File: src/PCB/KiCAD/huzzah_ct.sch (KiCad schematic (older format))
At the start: 6 parts, among them CON1 BARREL_JACK, U1 MCP3008, U2 DS18B20, U3 Adafruit_HUZZAH, U4 LM317T

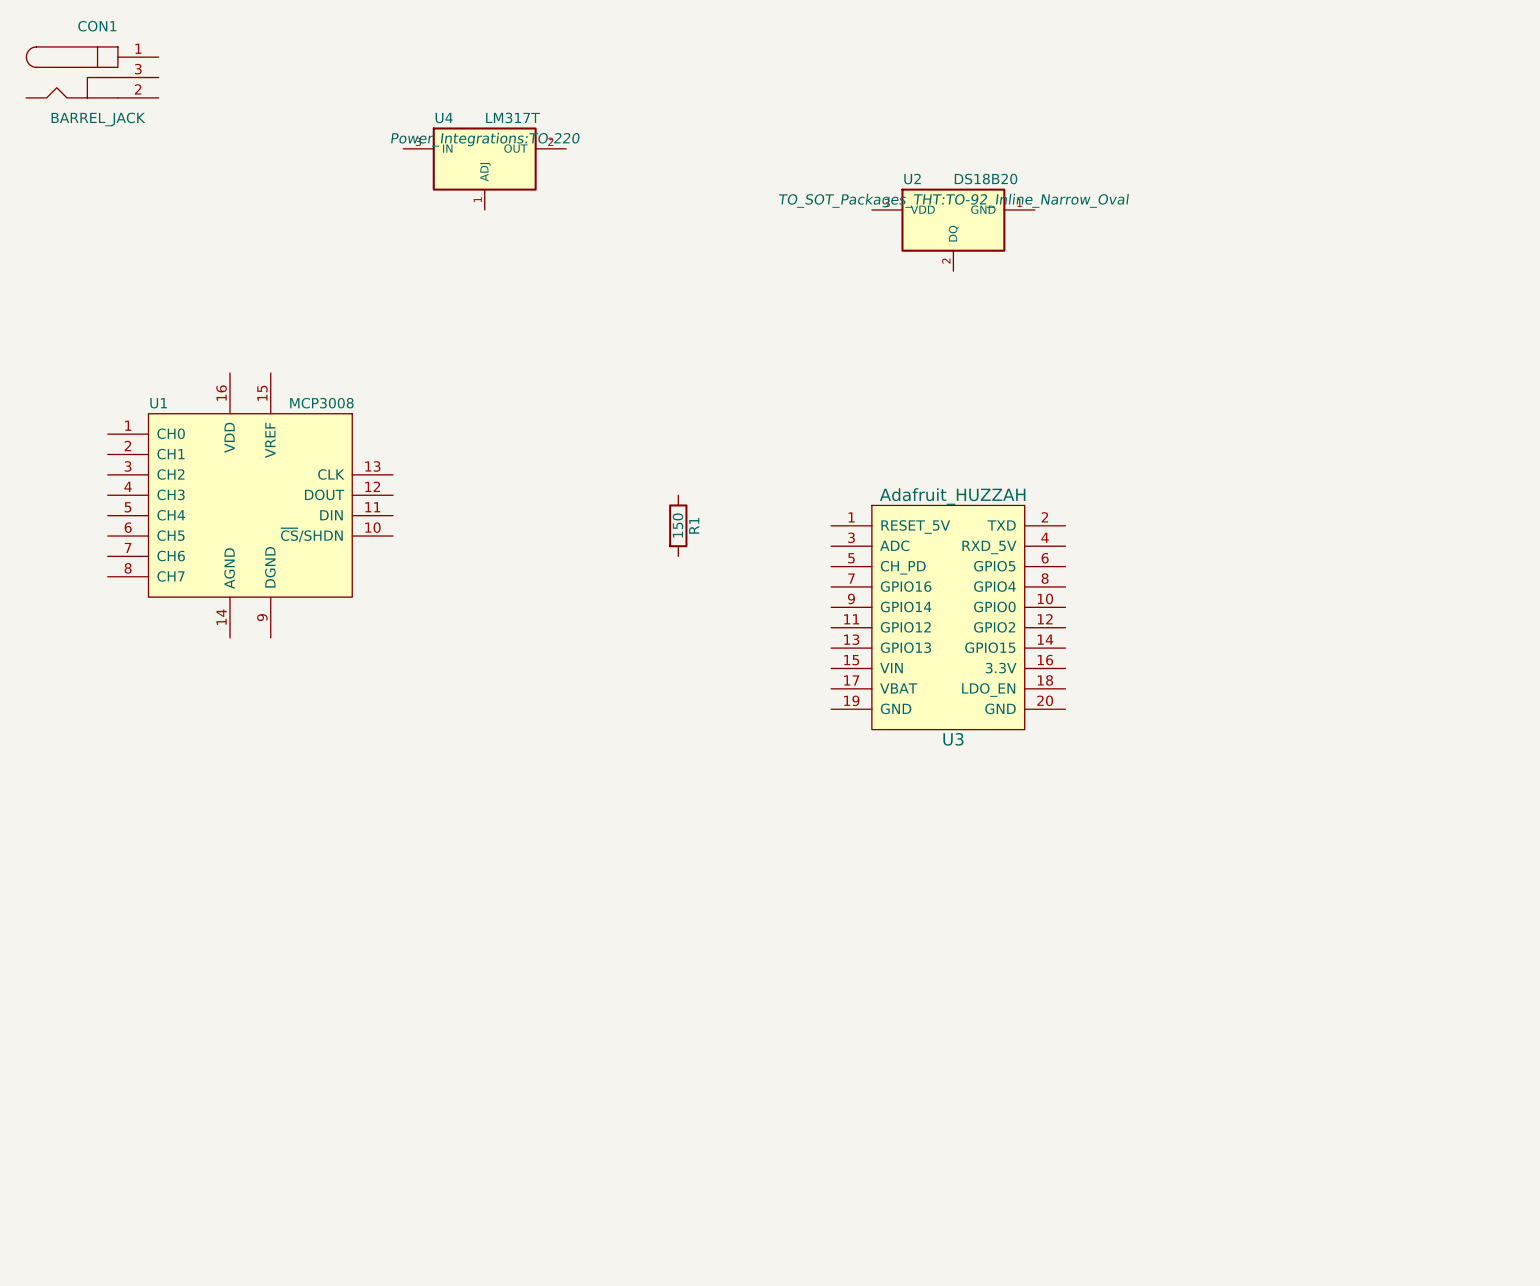
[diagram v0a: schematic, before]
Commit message: pcb routing
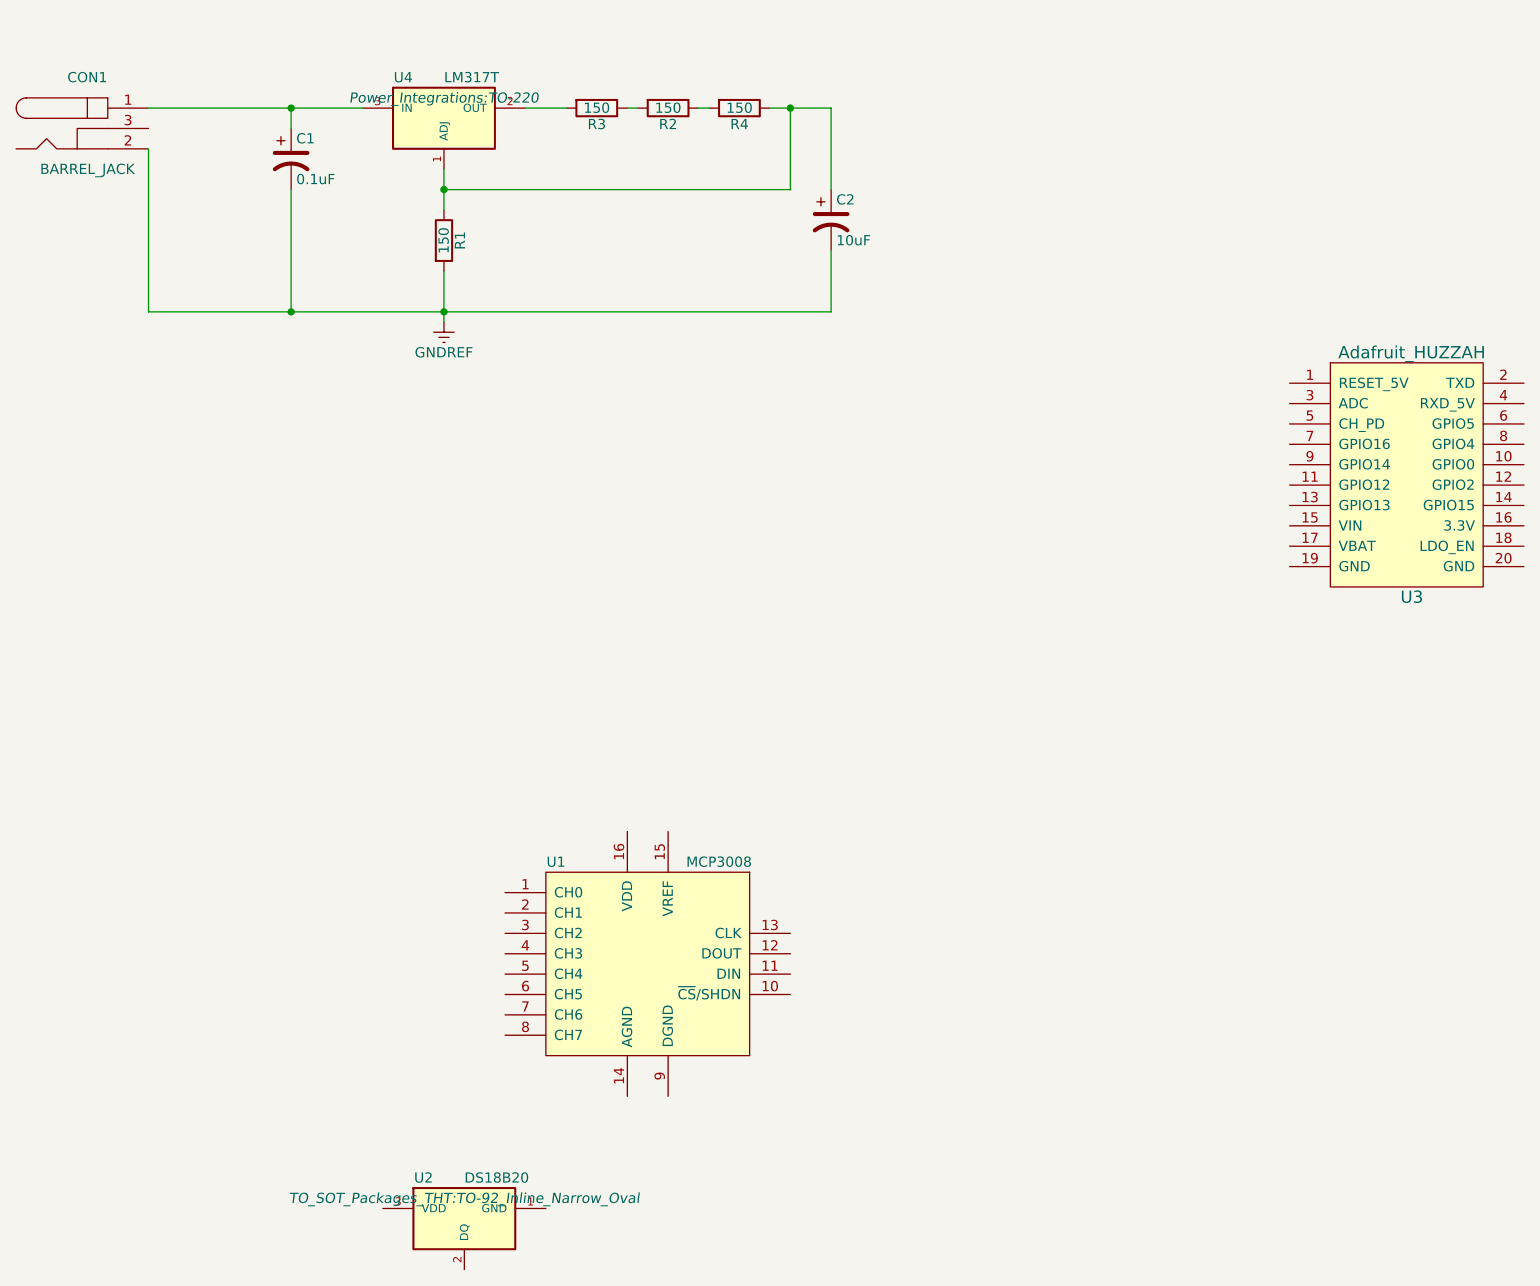
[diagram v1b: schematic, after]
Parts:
- added C1: 0.1uF, Capacitors_ThroughHole:C_Radial_D5_L11_P2, symbol CP1
- added C2: 10uF, Capacitors_ThroughHole:C_Radial_D5_L11_P2, symbol CP1
- added R2, R3, R4: 150, Resistors_ThroughHole:Resistor_Horizontal_RM7mm, symbol R
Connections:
- net at U4.1 (ADJ): now also R1.1, C2.1, R4.1
- net at U4.2 (OUT): now also R3.2
- net at U4.3 (IN): now also CON1.1, C1.1
- net GNDREF: now reaches CON1.2
- net GNDREF: now also R1.2, C1.2, C2.2
- new net: R2.1, R4.2
- new net: R2.2, R3.1
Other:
- moved on the sheet: CON1, R1, U1, U2, U3, U4
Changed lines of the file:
@@
 L Adafruit_HUZZAH U3
 U 1 1 56E6FE75
-P 5500 3750
-F 0 "U3" H 5500 3150 60  0000 C CNN
-F 1 "Adafruit_HUZZAH" H 5500 4350 60  0000 C CNN
-F 2 "Adafruit_huzzah:Adafruit HUZZAH" H 5400 3400 60  0001 C CNN
-F 3 "" H 5400 3400 60  0000 C CNN
-	1    5500 3750
+P 7750 3050
+F 0 "U3" H 7750 2450 60  0000 C CNN
+F 1 "Adafruit_HUZZAH" H 7750 3650 60  0000 C CNN
+F 2 "Adafruit_huzzah:Adafruit HUZZAH" H 7650 2700 60  0001 C CNN
+F 3 "" H 7650 2700 60  0000 C CNN
+	1    7750 3050
 	1    0    0    -1
 $EndComp
@@
 L MCP3008 U1
 U 1 1 56E6FF1E
-P 2050 3150
-F 0 "U1" H 1600 3600 50  0000 C CNN
-F 1 "MCP3008" H 2400 3600 50  0000 C CNN
-F 2 "Housings_DIP:DIP-16_W7.62mm" H 1950 3050 50  0001 C CNN
-F 3 "" H 2050 3150 50  0000 C CNN
-	1    2050 3150
+P 4000 5400
+F 0 "U1" H 3550 5850 50  0000 C CNN
+F 1 "MCP3008" H 4350 5850 50  0000 C CNN
+F 2 "Housings_DIP:DIP-16_W7.62mm" H 3900 5300 50  0001 C CNN
+F 3 "" H 4000 5400 50  0000 C CNN
+	1    4000 5400
 	1    0    0    -1
 $EndComp
@@
 L DS18B20 U2
 U 1 1 56E6FF7D
-P 5500 1800
-F 0 "U2" H 5300 2000 50  0000 C CNN
-F 1 "DS18B20" H 5500 2000 50  0000 L CNN
-F 2 "TO_SOT_Packages_THT:TO-92_Inline_Narrow_Oval" H 5500 1900 50  0000 C CIN
-F 3 "" H 5500 1800 50  0000 C CNN
-	1    5500 1800
+P 3100 6700
+F 0 "U2" H 2900 6900 50  0000 C CNN
+F 1 "DS18B20" H 3100 6900 50  0000 L CNN
+F 2 "TO_SOT_Packages_THT:TO-92_Inline_Narrow_Oval" H 3100 6800 50  0000 C CIN
+F 3 "" H 3100 6700 50  0000 C CNN
+	1    3100 6700
 	1    0    0    -1
 $EndComp
@@
 L LM317T U4
 U 1 1 56E70020
-P 3200 1500
-F 0 "U4" H 3000 1700 50  0000 C CNN
-F 1 "LM317T" H 3200 1700 50  0000 L CNN
-F 2 "Power_Integrations:TO-220" H 3200 1600 50  0000 C CIN
-F 3 "" H 3200 1500 50  0000 C CNN
-	1    3200 1500
+P 3000 1300
+F 0 "U4" H 2800 1500 50  0000 C CNN
+F 1 "LM317T" H 3000 1500 50  0000 L CNN
+F 2 "Power_Integrations:TO-220" H 3000 1400 50  0000 C CIN
+F 3 "" H 3000 1300 50  0000 C CNN
+	1    3000 1300
 	1    0    0    -1
 $EndComp
@@
 L BARREL_JACK CON1
 U 1 1 56E70131
-P 1300 1100
-F 0 "CON1" H 1300 1350 50  0000 C CNN
-F 1 "BARREL_JACK" H 1300 900 50  0000 C CNN
-F 2 "Connect:JACK_ALIM" H 1300 1100 50  0001 C CNN
-F 3 "" H 1300 1100 50  0000 C CNN
-	1    1300 1100
+P 1250 1350
+F 0 "CON1" H 1250 1600 50  0000 C CNN
+F 1 "BARREL_JACK" H 1250 1150 50  0000 C CNN
+F 2 "Connect:JACK_ALIM" H 1250 1350 50  0001 C CNN
+F 3 "" H 1250 1350 50  0000 C CNN
+	1    1250 1350
 	1    0    0    -1
 $EndComp
@@
 L R R1
 U 1 1 56E70875
-P 4150 3300
-F 0 "R1" V 4230 3300 50  0000 C CNN
-F 1 "150" V 4150 3300 50  0000 C CNN
-F 2 "Resistors_ThroughHole:Resistor_Horizontal_RM7mm" V 4080 3300 50  0001 C CNN
-F 3 "" H 4150 3300 50  0000 C CNN
-	1    4150 3300
+P 3000 1900
+F 0 "R1" V 3080 1900 50  0000 C CNN
+F 1 "150" V 3000 1900 50  0000 C CNN
+F 2 "Resistors_ThroughHole:Resistor_Horizontal_RM7mm" V 2930 1900 50  0001 C CNN
+F 3 "" H 3000 1900 50  0000 C CNN
+	1    3000 1900
 	1    0    0    -1
 $EndComp
+$Comp
+L CP1 C2
+U 1 1 56E71E56
+P 4900 1800
+F 0 "C2" H 4925 1900 50  0000 L CNN
+F 1 "10uF" H 4925 1700 50  0000 L CNN
+F 2 "Capacitors_ThroughHole:C_Radial_D5_L11_P2" H 4900 1800 50  0001 C CNN
+F 3 "" H 4900 1800 50  0000 C CNN
+	1    4900 1800
+	1    0    0    -1
+$EndComp
+$Comp
+L CP1 C1
+U 1 1 56E72069
+P 2250 1500
+F 0 "C1" H 2275 1600 50  0000 L CNN
+F 1 "0.1uF" H 2275 1400 50  0000 L CNN
+F 2 "Capacitors_ThroughHole:C_Radial_D5_L11_P2" H 2250 1500 50  0001 C CNN
+F 3 "" H 2250 1500 50  0000 C CNN
+	1    2250 1500
+	1    0    0    -1
+$EndComp
+$Comp
+L R R2
+U 1 1 56E72C3E
+P 4100 1250
+F 0 "R2" V 4180 1250 50  0000 C CNN
+F 1 "150" V 4100 1250 50  0000 C CNN
+F 2 "Resistors_ThroughHole:Resistor_Horizontal_RM7mm" V 4030 1250 50  0001 C CNN
+F 3 "" H 4100 1250 50  0000 C CNN
+	1    4100 1250
+	0    1    1    0
+$EndComp
+$Comp
+L R R3
+U 1 1 56E72C6F
+P 3750 1250
+F 0 "R3" V 3830 1250 50  0000 C CNN
+F 1 "150" V 3750 1250 50  0000 C CNN
+F 2 "Resistors_ThroughHole:Resistor_Horizontal_RM7mm" V 3680 1250 50  0001 C CNN
+F 3 "" H 3750 1250 50  0000 C CNN
+	1    3750 1250
+	0    1    1    0
+$EndComp
+$Comp
+L R R4
+U 1 1 56E72CB5
+P 4450 1250
+F 0 "R4" V 4530 1250 50  0000 C CNN
+F 1 "150" V 4450 1250 50  0000 C CNN
+F 2 "Resistors_ThroughHole:Resistor_Horizontal_RM7mm" V 4380 1250 50  0001 C CNN
+F 3 "" H 4450 1250 50  0000 C CNN
+	1    4450 1250
+	0    1    1    0
+$EndComp
+$Comp
+L GNDREF #PWR01
+U 1 1 56E7309D
+P 3000 2300
+F 0 "#PWR01" H 3000 2050 50  0001 C CNN
+F 1 "GNDREF" H 3000 2150 50  0000 C CNN
+F 2 "" H 3000 2300 50  0000 C CNN
+F 3 "" H 3000 2300 50  0000 C CNN
+	1    3000 2300
+	1    0    0    -1
+$EndComp
+Wire Wire Line
+	3000 1550 3000 1750
+Wire Wire Line
+	3000 2050 3000 2300
+Wire Wire Line
+	2600 1250 1550 1250
+Wire Wire Line
+	2250 1350 2250 1250
+Connection ~ 2250 1250
+Wire Wire Line
+	2250 1650 2250 2250
+Connection ~ 3000 2250
+Wire Wire Line
+	1550 1450 1550 2250
+Connection ~ 2250 2250
+Wire Wire Line
+	3400 1250 3600 1250
+Wire Wire Line
+	3900 1250 3950 1250
+Wire Wire Line
+	4250 1250 4300 1250
+Wire Wire Line
+	4600 1250 4900 1250
+Wire Wire Line
+	4900 1250 4900 1650
+Connection ~ 4700 1250
+Wire Wire Line
+	4700 1250 4700 1650
+Wire Wire Line
+	4700 1650 3000 1650
+Connection ~ 3000 1650
+Wire Wire Line
+	1550 2250 4900 2250
+Wire Wire Line
+	4900 2250 4900 1950
 $EndSCHEMATC
